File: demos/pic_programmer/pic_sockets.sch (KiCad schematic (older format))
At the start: 7 parts, among them P2 SUPP28, P3 SUPP40, U1 24Cxx, U5 PIC_18_PINS, U6 PIC_8_PINS

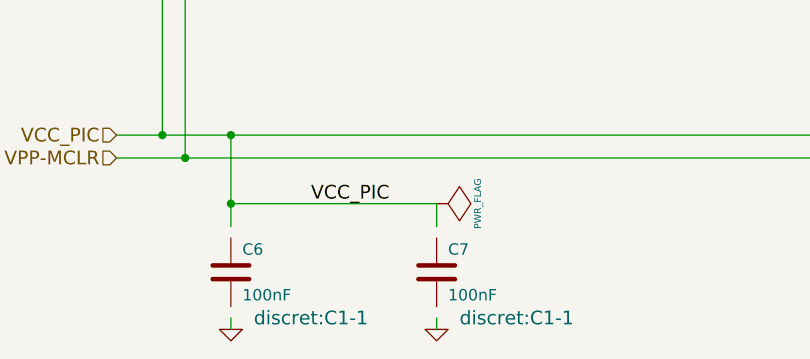
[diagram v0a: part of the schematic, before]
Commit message: merge from production bzr6934 to bzr 6953
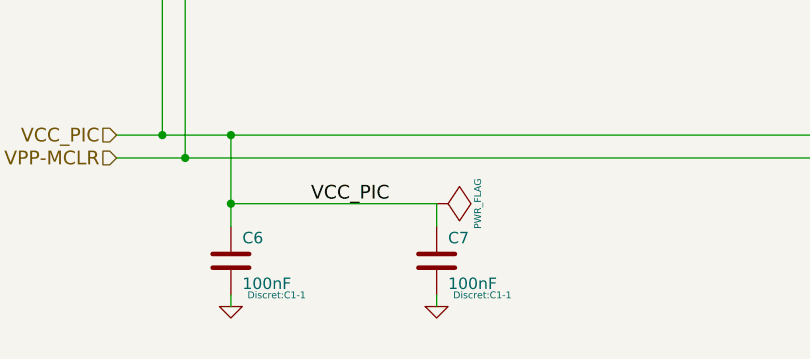
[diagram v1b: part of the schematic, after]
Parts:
- C6, C7: footprint discret:C1-1 -> Discret:C1-1
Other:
- moved on the sheet: C6, C7
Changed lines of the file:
@@
 EESchema Schematic File Version 2
+LIBS:device
 LIBS:pic_programmer_schlib
 LIBS:power
@@
 L GND #PWR040
 U 1 1 442AA147
-P 3300 7050
-F 0 "#PWR040" H 3300 7050 30  0001 C CNN
-F 1 "GND" H 3300 6980 30  0001 C CNN
-F 2 "" H 3300 7050 60  0001 C CNN
-F 3 "" H 3300 7050 60  0001 C CNN
-	1    3300 7050
+P 3300 6950
+F 0 "#PWR040" H 3300 6950 30  0001 C CNN
+F 1 "GND" H 3300 6880 30  0001 C CNN
+F 2 "" H 3300 6950 60  0001 C CNN
+F 3 "" H 3300 6950 60  0001 C CNN
+	1    3300 6950
 	1    0    0    -1
 $EndComp
@@
 L C C7
 U 1 1 442AA145
-P 3300 6800
-F 0 "C7" H 3350 6900 50  0000 L CNN
-F 1 "100nF" H 3350 6700 50  0000 L CNN
-F 2 "discret:C1-1" H 3650 6600 60  0000 C CNN
-F 3 "" H 3300 6800 60  0001 C CNN
-	1    3300 6800
+P 3300 6750
+F 0 "C7" H 3350 6850 50  0000 L CNN
+F 1 "100nF" H 3350 6650 50  0000 L CNN
+F 2 "Discret:C1-1" H 3500 6600 30  0000 C CNN
+F 3 "" H 3300 6750 60  0001 C CNN
+	1    3300 6750
 	1    0    0    -1
 $EndComp
@@
 L GND #PWR041
 U 1 1 442AA138
-P 2400 7050
-F 0 "#PWR041" H 2400 7050 30  0001 C CNN
-F 1 "GND" H 2400 6980 30  0001 C CNN
-F 2 "" H 2400 7050 60  0001 C CNN
-F 3 "" H 2400 7050 60  0001 C CNN
-	1    2400 7050
+P 2400 6950
+F 0 "#PWR041" H 2400 6950 30  0001 C CNN
+F 1 "GND" H 2400 6880 30  0001 C CNN
+F 2 "" H 2400 6950 60  0001 C CNN
+F 3 "" H 2400 6950 60  0001 C CNN
+	1    2400 6950
 	1    0    0    -1
 $EndComp
@@
 L C C6
 U 1 1 442AA12B
-P 2400 6800
-F 0 "C6" H 2450 6900 50  0000 L CNN
-F 1 "100nF" H 2450 6700 50  0000 L CNN
-F 2 "discret:C1-1" H 2750 6600 60  0000 C CNN
-F 3 "" H 2400 6800 60  0001 C CNN
-	1    2400 6800
+P 2400 6750
+F 0 "C6" H 2450 6850 50  0000 L CNN
+F 1 "100nF" H 2450 6650 50  0000 L CNN
+F 2 "Discret:C1-1" H 2600 6600 30  0000 C CNN
+F 3 "" H 2400 6750 60  0001 C CNN
+	1    2400 6750
 	1    0    0    -1
 $EndComp
@@
 	3700 1850 3700 1800
 Wire Wire Line
-	2400 7000 2400 7050
-Wire Wire Line
-	3300 7000 3300 7050
+	2400 6900 2400 6950
+Wire Wire Line
+	3300 6900 3300 6950
 $Comp
 L PWR_FLAG #FLG047
